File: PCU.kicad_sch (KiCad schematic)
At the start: 7 parts, among them U4 EPC2152, Y1 AMDLA4020S-220MT

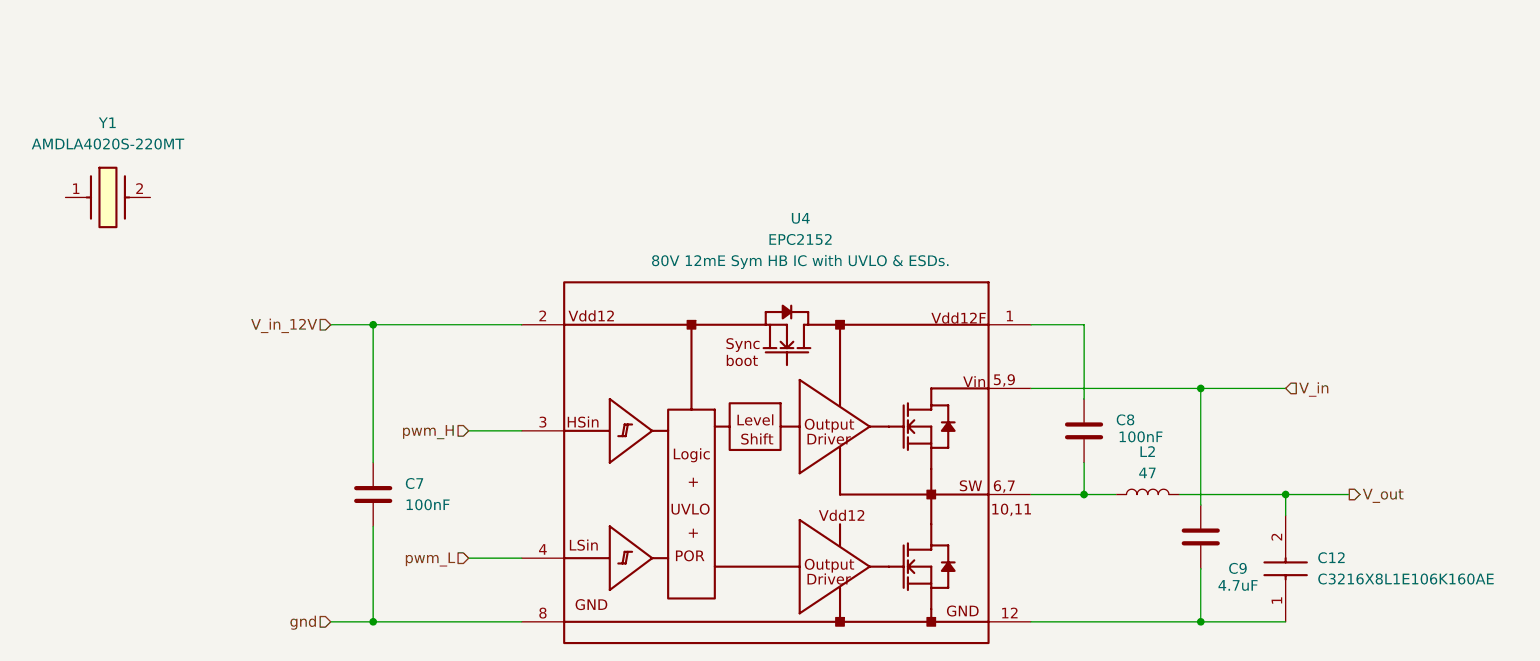
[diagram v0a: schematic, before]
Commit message: lastest
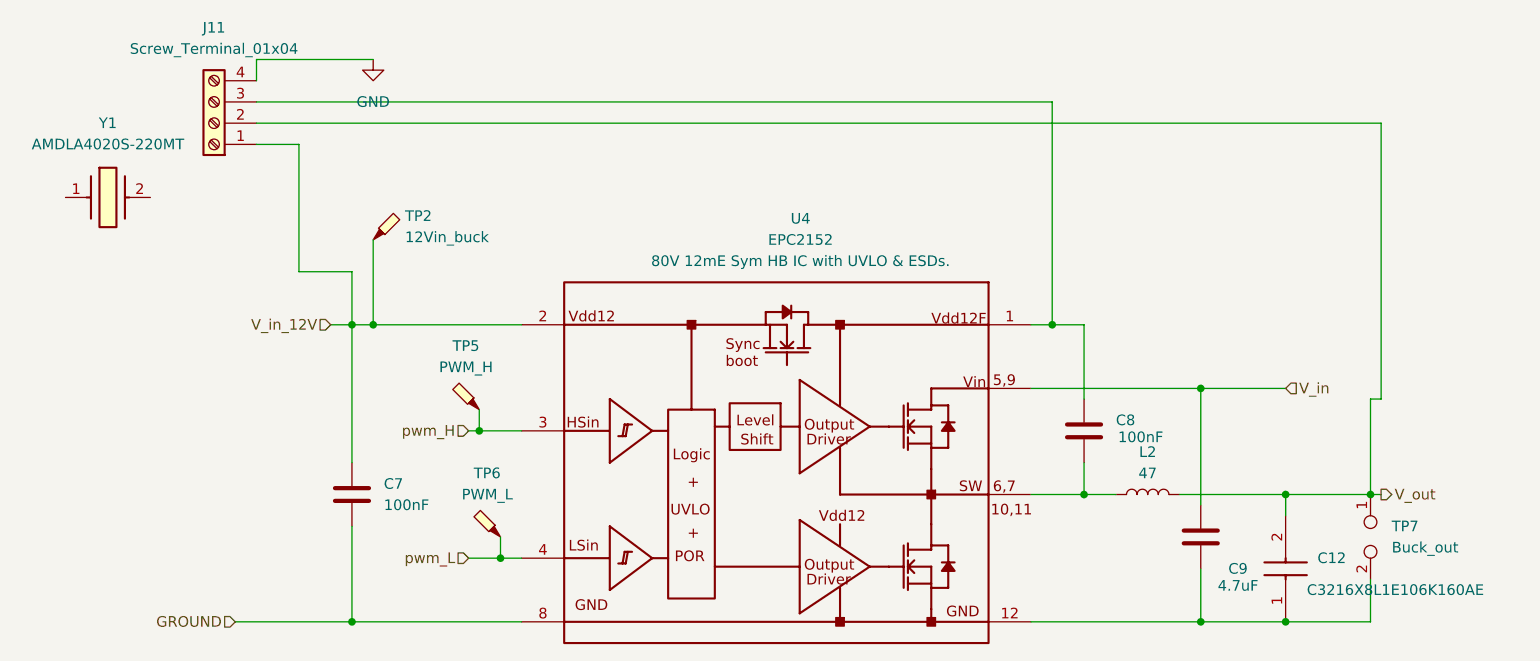
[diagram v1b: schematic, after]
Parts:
- added J11: Screw_Terminal_01x04, TerminalBlock_Phoenix:TerminalBlock_Phoenix_MKDS-1,5-4-5.08_1x04_P5.08mm_Horizontal, symbol Connector:Screw_Terminal_01x04
- added TP2: 12Vin_buck, TestPoint:TestPoint_Pad_D2.0mm, symbol Connector:TestPoint_Probe
- added TP5: PWM_H, TestPoint:TestPoint_Pad_D2.0mm, symbol Connector:TestPoint_Probe
- added TP6: PWM_L, TestPoint:TestPoint_Pad_D2.0mm, symbol Connector:TestPoint_Probe
- added TP7: Buck_out, TestPoint:TestPoint_Pad_D2.0mm, symbol Connector:TestPoint_2Pole
- C12: footprint CAPC3216X180N -> PULSE_Library:CAPC3216X180N
- C7, C8, C9: footprint (none) -> Capacitor_SMD:C_0201_0603Metric
- L2: footprint (none) -> Inductor_SMD:L_10.4x10.4_H4.8
- U4: footprint EPC_FETs:D0122 -> PULSE_Library:VREG_EPC2152ENGRT
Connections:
- net V_in_12V: now also J11.1 (Pin_1), TP2.1
- net V_out: now also J11.2 (Pin_2), TP7.1
- net pwm_H: now also TP5.1
- net pwm_L: now also TP6.1
- net at C12.1, C9.2, U4.12 (Vss): now also TP7.2
- net at C8.1, U4.1 (Vdd12F): now also J11.3 (Pin_3)
- net gnd renamed GROUND
- new net GND: J11.4 (Pin_4)
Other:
- moved on the sheet: C7
